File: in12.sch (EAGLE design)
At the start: 34 parts, among them U1 MICROCHIP_HV5622PG-GMICROCHIP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, U2 MICROCHIP_HV5622PG-GMICROCHIP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, U3 MICROCHIP_HV5622PG-GMICROCHIP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

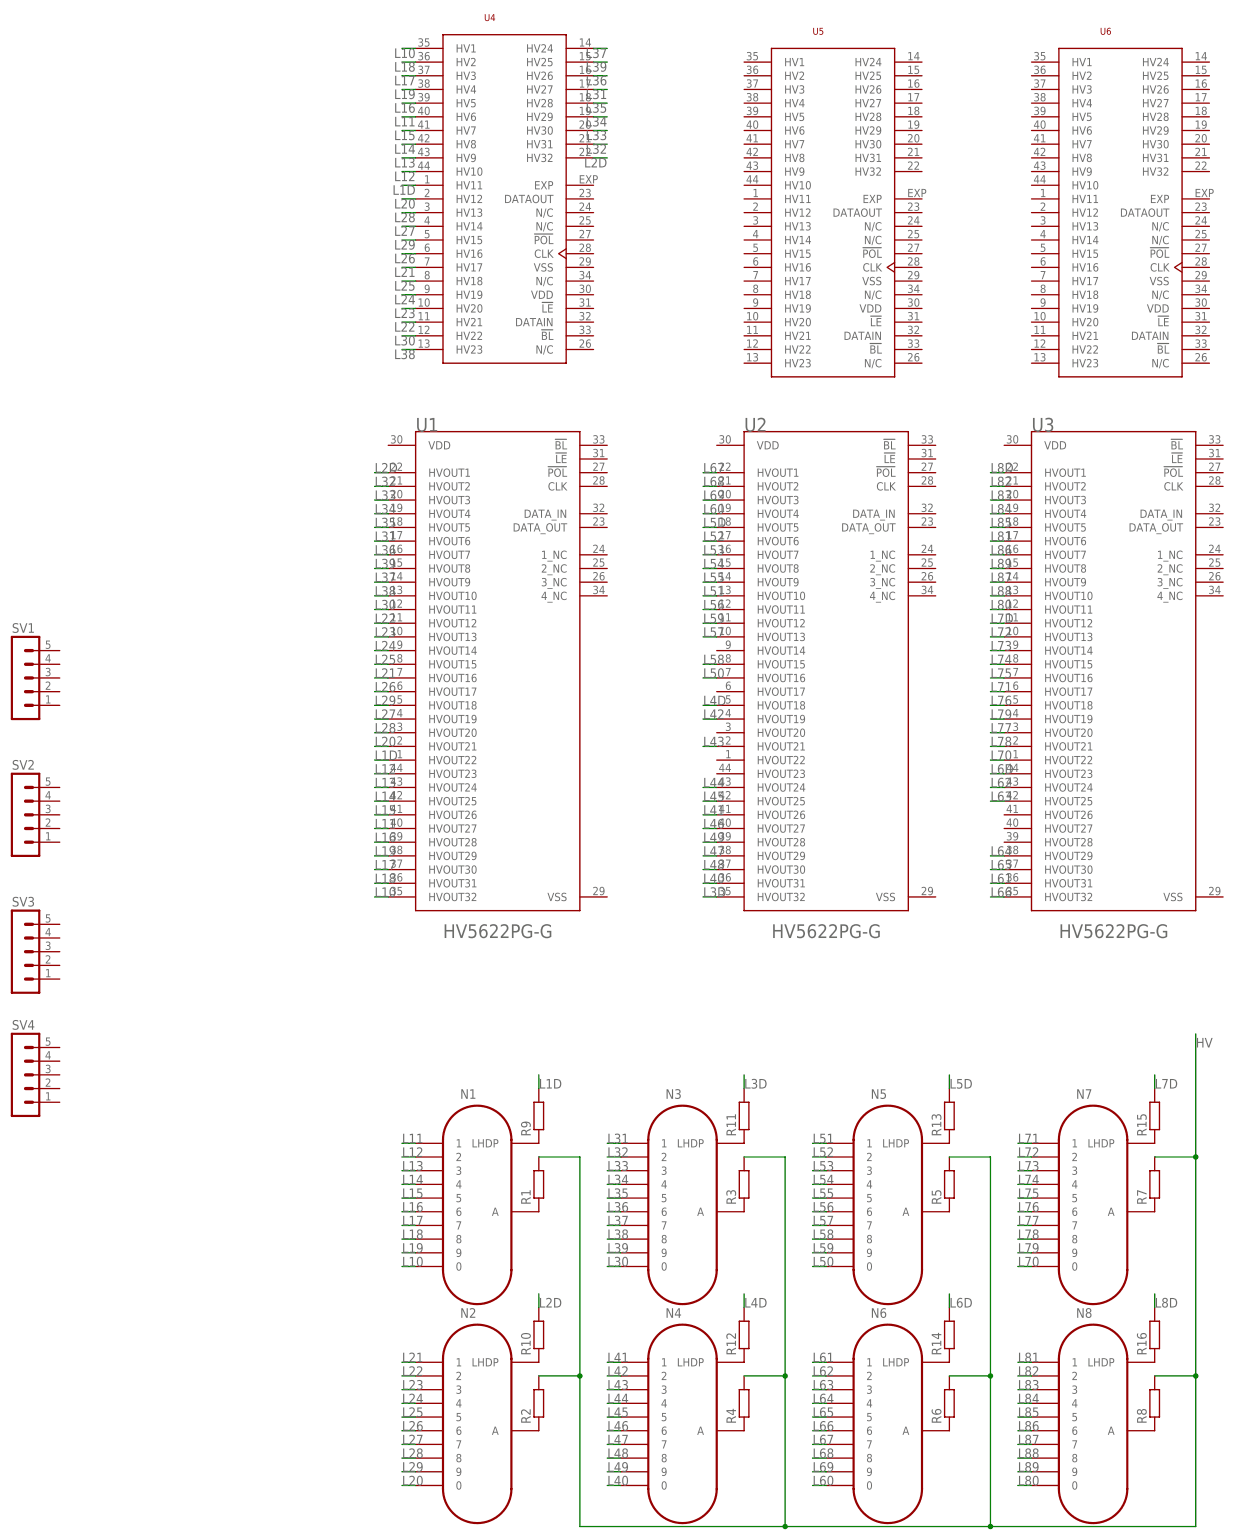
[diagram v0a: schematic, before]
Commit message: 5523 still need shuffle pins
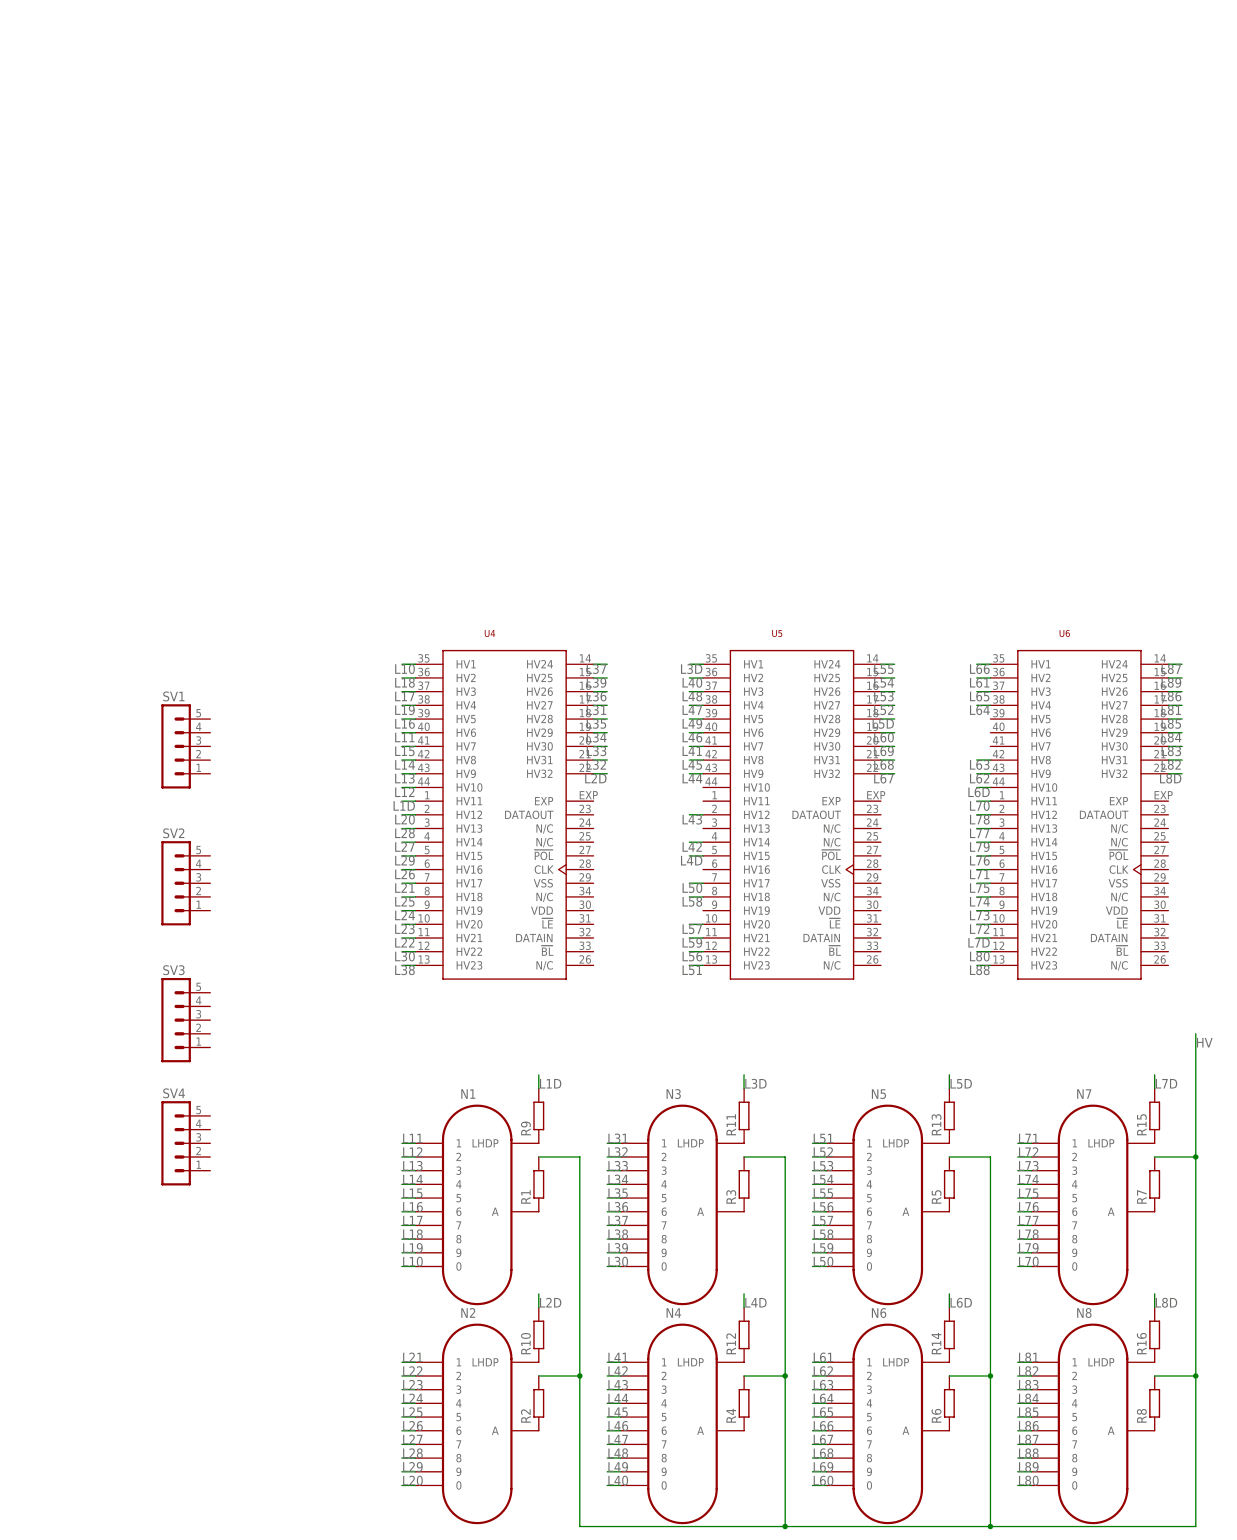
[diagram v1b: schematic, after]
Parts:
- removed U1, U2, U3: MICROCHIP_HV5622PG-GMICROCHIP_HV5622PG-G_0_0, Microchip - HV5622PG-G:MICROCHIP_HV5622PG-GMICROCHIP_HV5622PG-G_0_0
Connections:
- net L10: no longer U1.HVOUT32
- net L11: no longer U1.HVOUT27
- net L12: no longer U1.HVOUT23
- net L13: no longer U1.HVOUT24
- net L14: no longer U1.HVOUT25
- net L15: no longer U1.HVOUT26
- net L16: no longer U1.HVOUT28
- net L17: no longer U1.HVOUT30
- net L18: no longer U1.HVOUT31
- net L19: no longer U1.HVOUT29
- net L1D: no longer U1.HVOUT22
- net L20: no longer U1.HVOUT21
- net L21: no longer U1.HVOUT16
- net L22: no longer U1.HVOUT12
- net L23: no longer U1.HVOUT13
- net L24: no longer U1.HVOUT14
- net L25: no longer U1.HVOUT15
- net L26: no longer U1.HVOUT17
- net L27: no longer U1.HVOUT19
- net L28: no longer U1.HVOUT20
- net L29: no longer U1.HVOUT18
- net L2D: no longer U1.HVOUT1
- net L30: no longer U1.HVOUT11
- net L31: no longer U1.HVOUT6
- net L32: no longer U1.HVOUT2
- net L33: no longer U1.HVOUT3
- net L34: no longer U1.HVOUT4
- net L35: no longer U1.HVOUT5
- net L36: no longer U1.HVOUT7
- net L37: no longer U1.HVOUT9
- net L38: no longer U1.HVOUT10
- net L39: no longer U1.HVOUT8
- net L3D: now also U5.HV1; no longer U2.HVOUT32
- net L40: now also U5.HV2; no longer U2.HVOUT31
- net L41: now also U5.HV7; no longer U2.HVOUT26
- net L42: now also U5.HV14; no longer U2.HVOUT19
- net L43: now also U5.HV12; no longer U2.HVOUT21
- net L44: now also U5.HV9; no longer U2.HVOUT24
- net L45: now also U5.HV8; no longer U2.HVOUT25
- net L46: now also U5.HV6; no longer U2.HVOUT27
- net L47: now also U5.HV4; no longer U2.HVOUT29
- net L48: now also U5.HV3; no longer U2.HVOUT30
- net L49: now also U5.HV5; no longer U2.HVOUT28
- net L4D: now also U5.HV15; no longer U2.HVOUT18
- net L50: now also U5.HV17; no longer U2.HVOUT16
- net L51: now also U5.HV23; no longer U2.HVOUT10
- net L52: now also U5.HV27; no longer U2.HVOUT6
- net L53: now also U5.HV26; no longer U2.HVOUT7
- net L54: now also U5.HV25; no longer U2.HVOUT8
- net L55: now also U5.HV24; no longer U2.HVOUT9
- net L56: now also U5.HV22; no longer U2.HVOUT11
- net L57: now also U5.HV20; no longer U2.HVOUT13
- net L58: now also U5.HV18; no longer U2.HVOUT15
- net L59: now also U5.HV21; no longer U2.HVOUT12
- net L5D: now also U5.HV28; no longer U2.HVOUT5
- net L60: now also U5.HV29; no longer U2.HVOUT4
- net L61: now also U6.HV2; no longer U3.HVOUT31
- net L62: now also U6.HV9; no longer U3.HVOUT24
- net L63: now also U6.HV8; no longer U3.HVOUT25
- net L64: now also U6.HV4; no longer U3.HVOUT29
- net L65: now also U6.HV3; no longer U3.HVOUT30
- net L66: now also U6.HV1; no longer U3.HVOUT32
- net L67: now also U5.HV32; no longer U2.HVOUT1
- net L68: now also U5.HV31; no longer U2.HVOUT2
- net L69: now also U5.HV30; no longer U2.HVOUT3
- net L6D: now also U6.HV10; no longer U3.HVOUT23
- net L70: now also U6.HV11; no longer U3.HVOUT22
- net L71: now also U6.HV16; no longer U3.HVOUT17
- net L72: now also U6.HV20; no longer U3.HVOUT13
- net L73: now also U6.HV19; no longer U3.HVOUT14
- net L74: now also U6.HV18; no longer U3.HVOUT15
- net L75: now also U6.HV17; no longer U3.HVOUT16
- net L76: now also U6.HV15; no longer U3.HVOUT18
- net L77: now also U6.HV13; no longer U3.HVOUT20
- net L78: now also U6.HV12; no longer U3.HVOUT21
- net L79: now also U6.HV14; no longer U3.HVOUT19
- net L7D: now also U6.HV21; no longer U3.HVOUT12
- net L80: now also U6.HV22; no longer U3.HVOUT11
- net L81: now also U6.HV27; no longer U3.HVOUT6
- net L82: now also U6.HV31; no longer U3.HVOUT2
- net L83: now also U6.HV30; no longer U3.HVOUT3
- net L84: now also U6.HV29; no longer U3.HVOUT4
- net L85: now also U6.HV28; no longer U3.HVOUT5
- net L86: now also U6.HV26; no longer U3.HVOUT7
- net L87: now also U6.HV24; no longer U3.HVOUT9
- net L88: now also U6.HV23; no longer U3.HVOUT10
- net L89: now also U6.HV25; no longer U3.HVOUT8
- net L8D: now also U6.HV32; no longer U3.HVOUT1
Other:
- moved on the sheet: SV1, SV2, SV3, SV4, U4, U5, U6
